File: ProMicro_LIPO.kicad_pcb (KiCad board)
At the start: 2 copper layers, 17.8 x 27.9 mm, 25 parts, among them J1 JST, U1 MCP73831-2-OT, U2 TPS61090

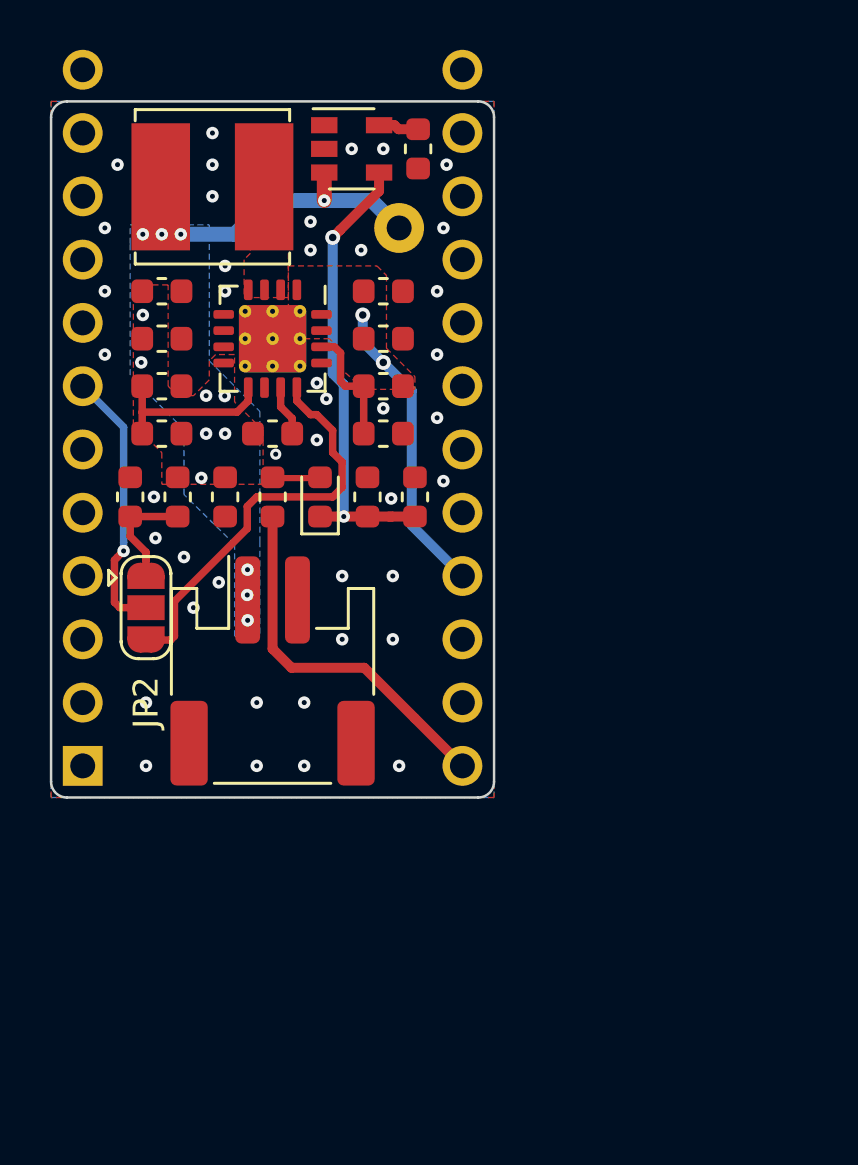
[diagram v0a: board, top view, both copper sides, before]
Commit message: trigger CI run
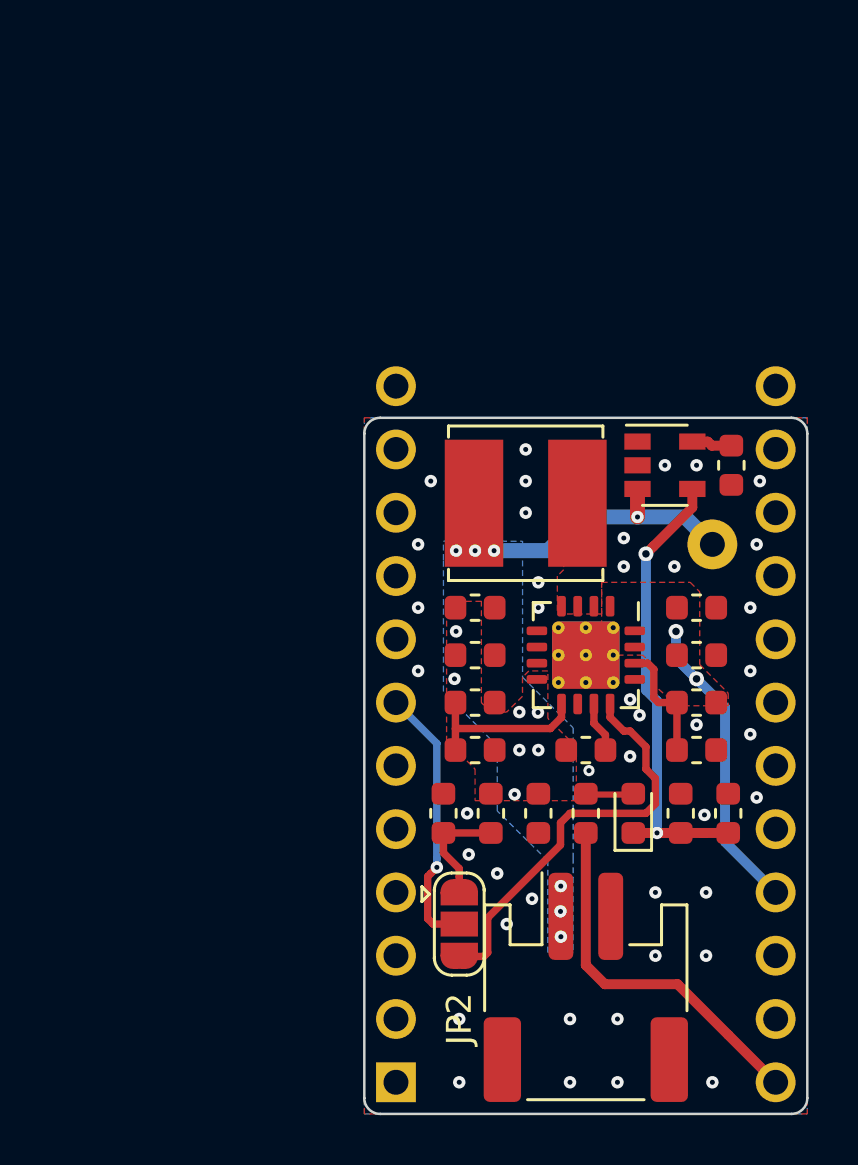
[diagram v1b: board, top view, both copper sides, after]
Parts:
- moved A1 17.9 mm to (63.4, 114.9)
- moved C1 17.9 mm to (74.8, 104.1)
- moved C3 17.9 mm to (66.5, 95.9)
- moved C4 17.9 mm to (66.5, 97.8)
- moved C6 17.9 mm to (75.4, 95.9)
- moved C7 17.9 mm to (75.4, 97.8)
- moved L1 17.9 mm to (68.6, 91.7)
- moved R1 17.9 mm to (67.2, 104.1)
- moved R2 17.9 mm to (65.3, 104.1)
- moved U1 17.9 mm to (74.2, 90.2)
- moved C2 17.9 mm to (76.7, 104.1)
- moved C5 17.9 mm to (69.1, 104.1)
- moved D1 17.9 mm to (72.9, 104.1)
- moved F1 17.9 mm to (71.0, 104.1)
- moved J1 17.9 mm to (71.0, 111.1)
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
